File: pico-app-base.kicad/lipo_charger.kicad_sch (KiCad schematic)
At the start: 13 parts, among them J7 JST-PH2 Bat, J9 Alt Bat, SW2 SW_ON, U3 MCP73831-2-OT, U4 XB6166IS

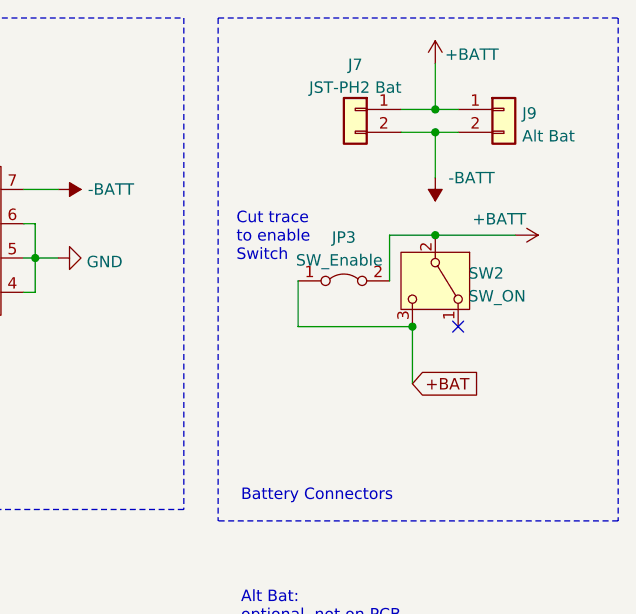
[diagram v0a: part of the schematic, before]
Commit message: added zones and connections
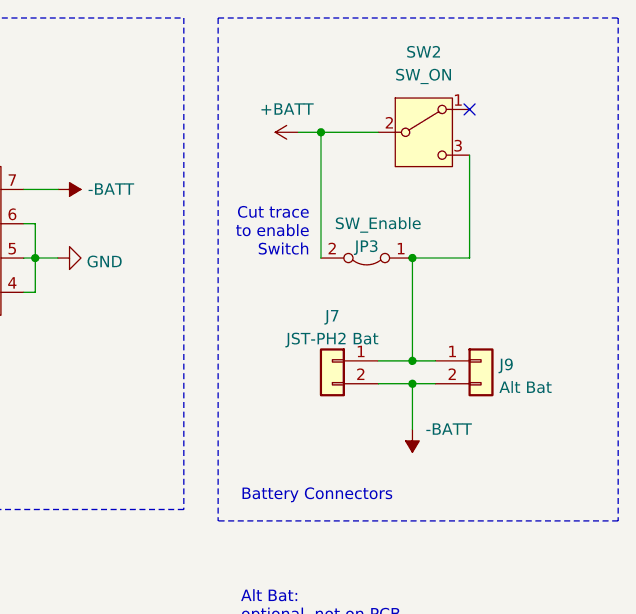
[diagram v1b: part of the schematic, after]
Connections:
- net +BATT: no longer J7.1 (Pin_1), J9.1 (Pin_1)
- net +BAT: no longer names the net of JP3.1 (A), SW2.3 (C)
- net +BAT: now also J7.1 (Pin_1), J9.1 (Pin_1)
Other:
- moved on the sheet: J7, J9, JP3, SW2
